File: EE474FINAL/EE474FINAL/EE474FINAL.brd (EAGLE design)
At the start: 69.5 x 84.8 mm, 61 parts, among them U1 TM4C123_DEVICE, U4 3.3V, Y1 32kHz, Y2 Y2

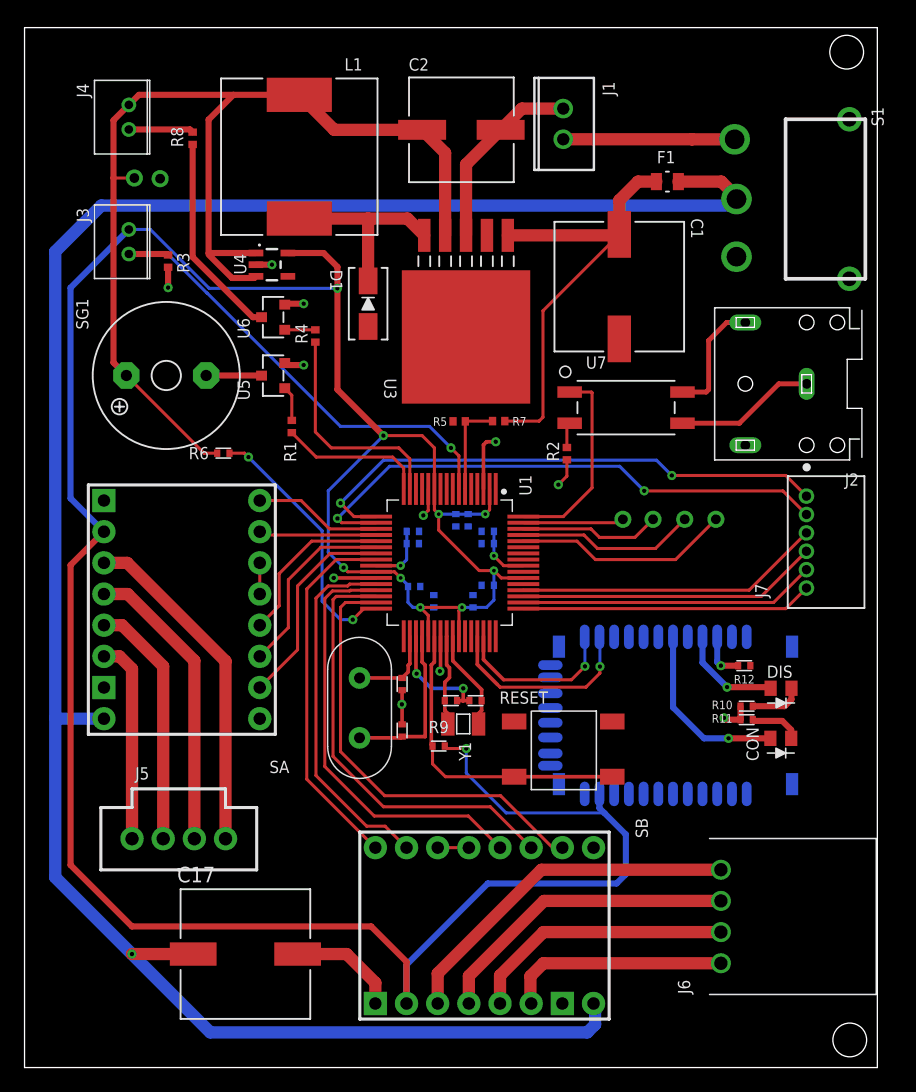
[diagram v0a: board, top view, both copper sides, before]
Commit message: done
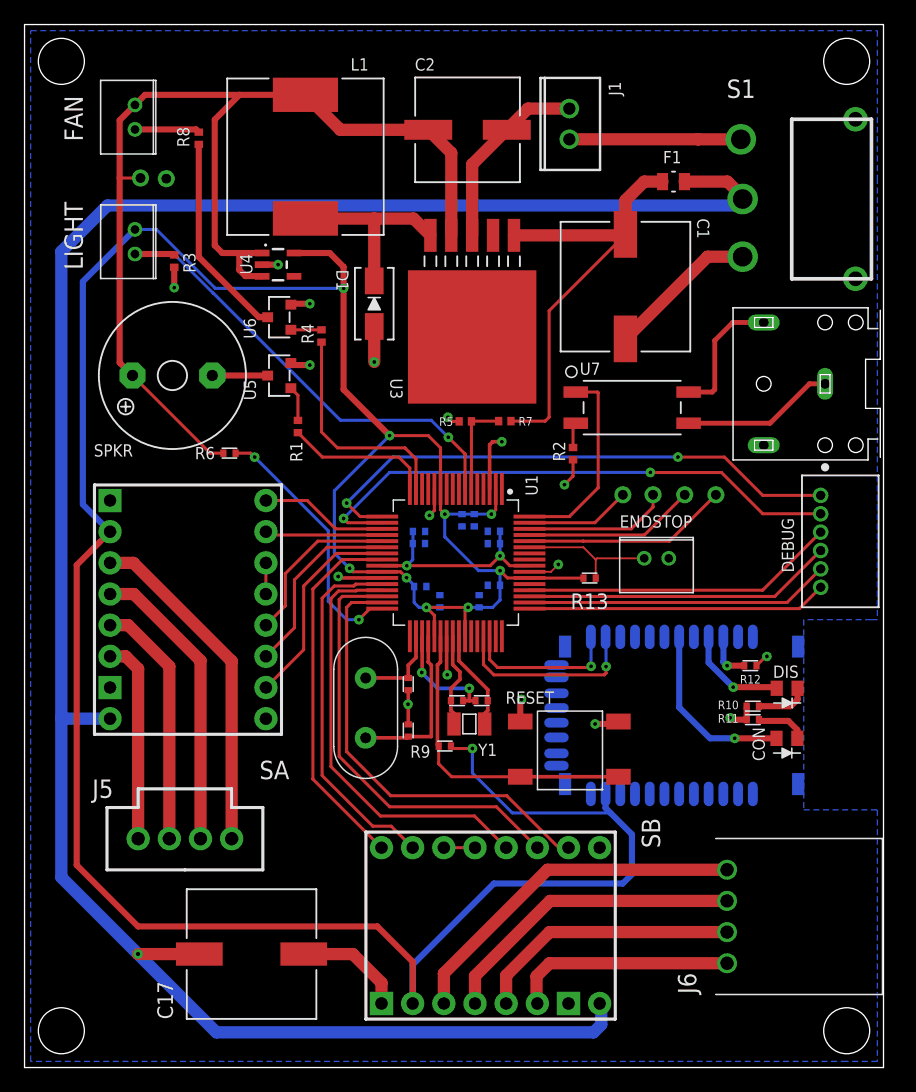
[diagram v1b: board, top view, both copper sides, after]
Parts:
- removed J3, J4: (no value), MICROCONTROLLER:2POS_JSTVERT_2.00
- removed J7: (no value), MICROCONTROLLER:6POS_JST
- removed SG1: F/QMBIII, buzzer:F/QMBIII
- added DEBUG: (no value), MICROCONTROLLER:6POS_JST
- added ENDSTOP, FAN, LIGHT: (no value), MICROCONTROLLER:2POS_JSTVERT_2.00
- added R13: (no value), MICROCONTROLLER:CAPC1005X35N
- added SPKR: F/QMBIII, buzzer:F/QMBIII
- added U$1: (no value), MICROCONTROLLER:LOGO_B
- moved PD0 2.00 mm to (53.8, 46.7)
- moved PD1 2.00 mm to (51.2, 46.7)
- moved PD2 2.00 mm to (48.8, 46.7)
- moved PE5 2.00 mm to (56.3, 46.7)
- moved J2 1.50 mm to (65.2, 55.7)
- moved C1 0.50 mm to (49.0, 63.6)
- moved C10 0.50 mm to (38.3, 42.7)
- moved C11 0.50 mm to (36.6, 44.6)
- moved C12 0.50 mm to (35.6, 44.6)
- moved C13 0.50 mm to (32.2, 39.2)
- moved C14 0.50 mm to (33.9, 38.0)
- moved C15 0.50 mm to (37.0, 38.0)
- moved C16 0.50 mm to (38.2, 39.3)
- moved C17 0.50 mm to (18.5, 9.25)
- moved C2 0.50 mm to (36.1, 76.4)
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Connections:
- new net N$15: ENDSTOP.1, R13.1, U1.59
- net +3V3: now also LIGHT.1, R13.2; no longer J3.1
- net +5V: now also FAN.1, SPKR.+; no longer J4.1, SG1.+
- net FAN_OUT: now also FAN.2; no longer J4.2
- net GND: now also ENDSTOP.2
- net LT: now also LIGHT.2; no longer J3.2
- net N$2: now also SPKR.-; no longer SG1.-
- net RXD: now also DEBUG.6; no longer J7.6
- net TCK: now also DEBUG.4; no longer J7.4
- net TDI: now also DEBUG.2; no longer J7.2
- net TDO: now also DEBUG.1; no longer J7.1
- net TMS: now also DEBUG.3; no longer J7.3
- net TXD: now also DEBUG.5; no longer J7.5
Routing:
- net GND: track 51.7 -> 76.2 mm, vias 11 -> 17
- net N$15: track 0.00 -> 11.3 mm
- net VDDC: track 9.73 -> 17.7 mm
- net +3V3: track 238.0 -> 243.6 mm
- net +5V: track 91.8 -> 90.2 mm
- net N$3: track 9.81 -> 10.8 mm
- net N$4: track 11.5 -> 12.5 mm
- net PE5: track 17.7 -> 16.8 mm
- net RXD: track 44.0 -> 44.8 mm
- net RX-1: track 13.7 -> 12.9 mm
- net TX-0: track 16.5 -> 15.7 mm
- net TMS: track 24.6 -> 25.3 mm
- net TDO: track 23.8 -> 24.4 mm
- net TCK: track 25.0 -> 25.7 mm
- net TDI: track 24.2 -> 24.9 mm
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- added copper zone on layer 16, net GND
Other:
- board size 69.5 x 84.8 mm -> 70 x 85 mm
- board text added: "BRANDON IAMS EE 474 FINAL PROJECT"

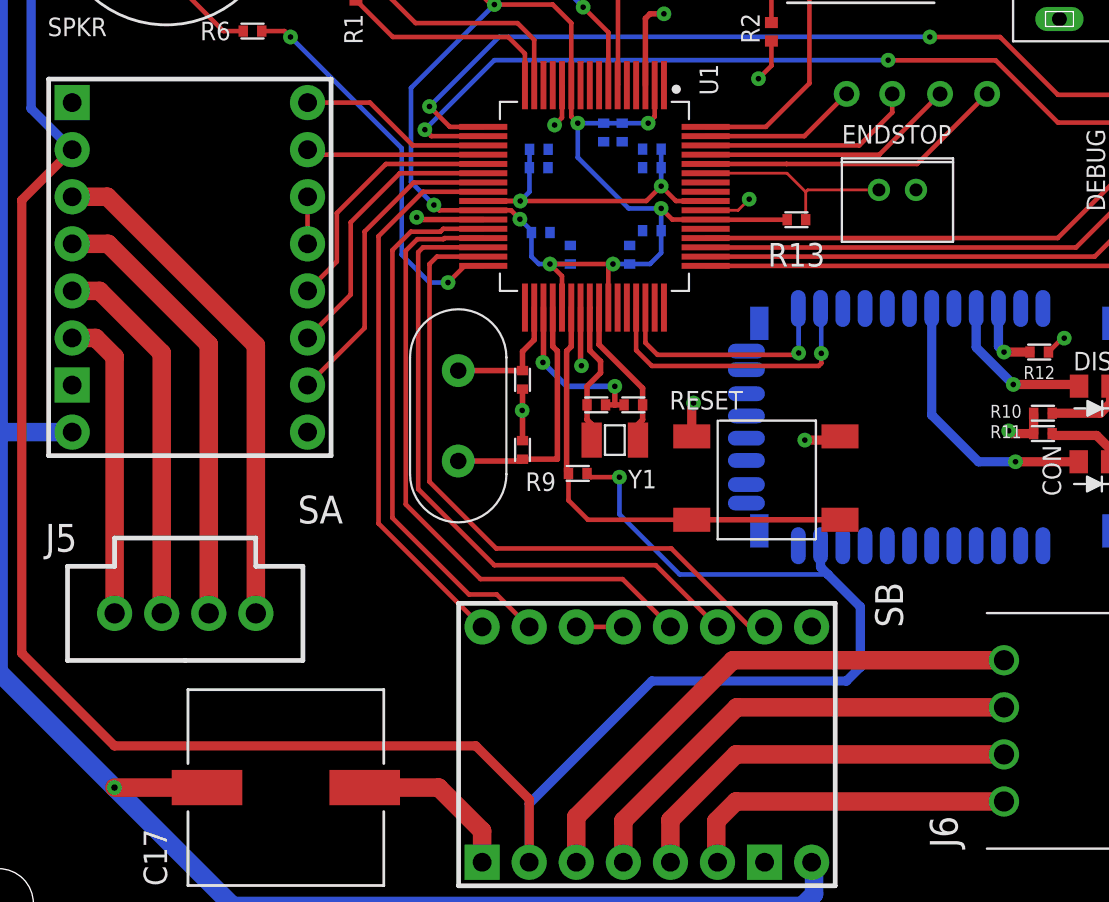
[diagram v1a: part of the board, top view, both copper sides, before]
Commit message: fixing...
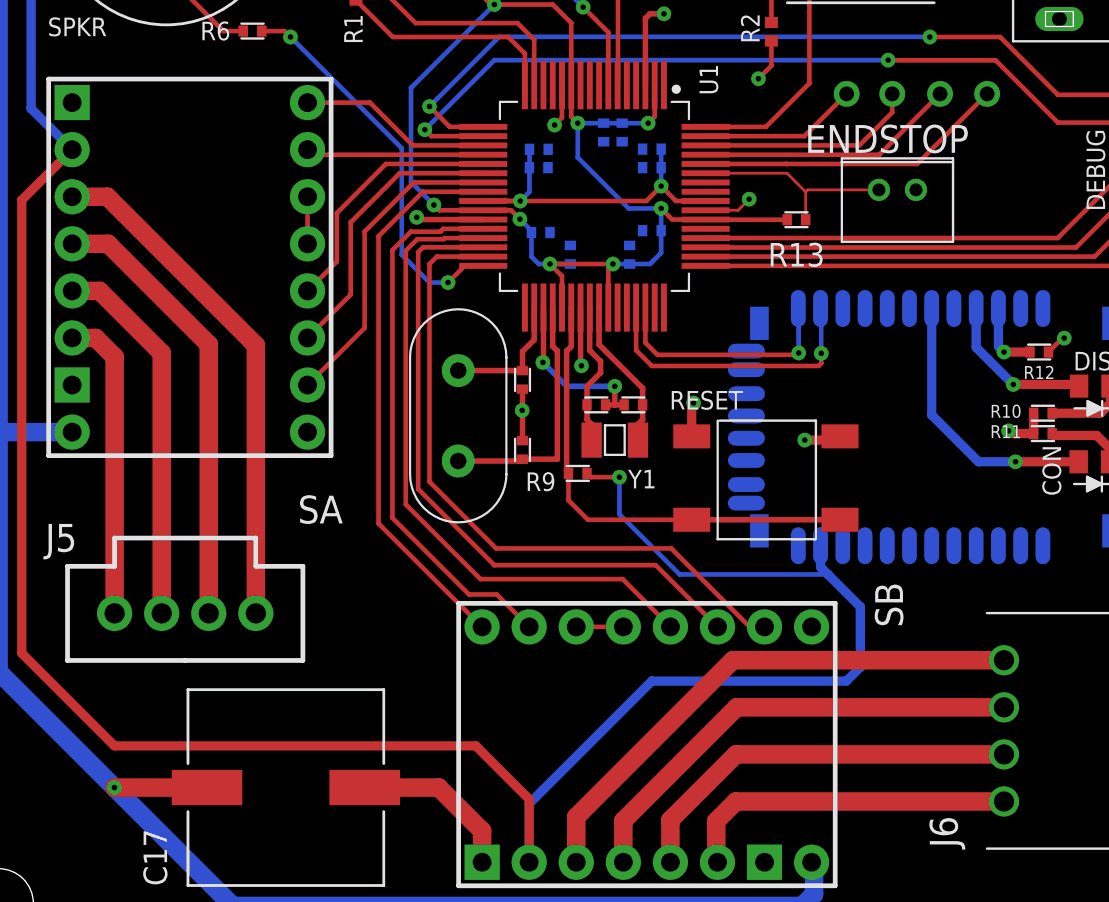
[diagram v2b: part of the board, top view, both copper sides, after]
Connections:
- net GND: now also U3.6

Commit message: merge :
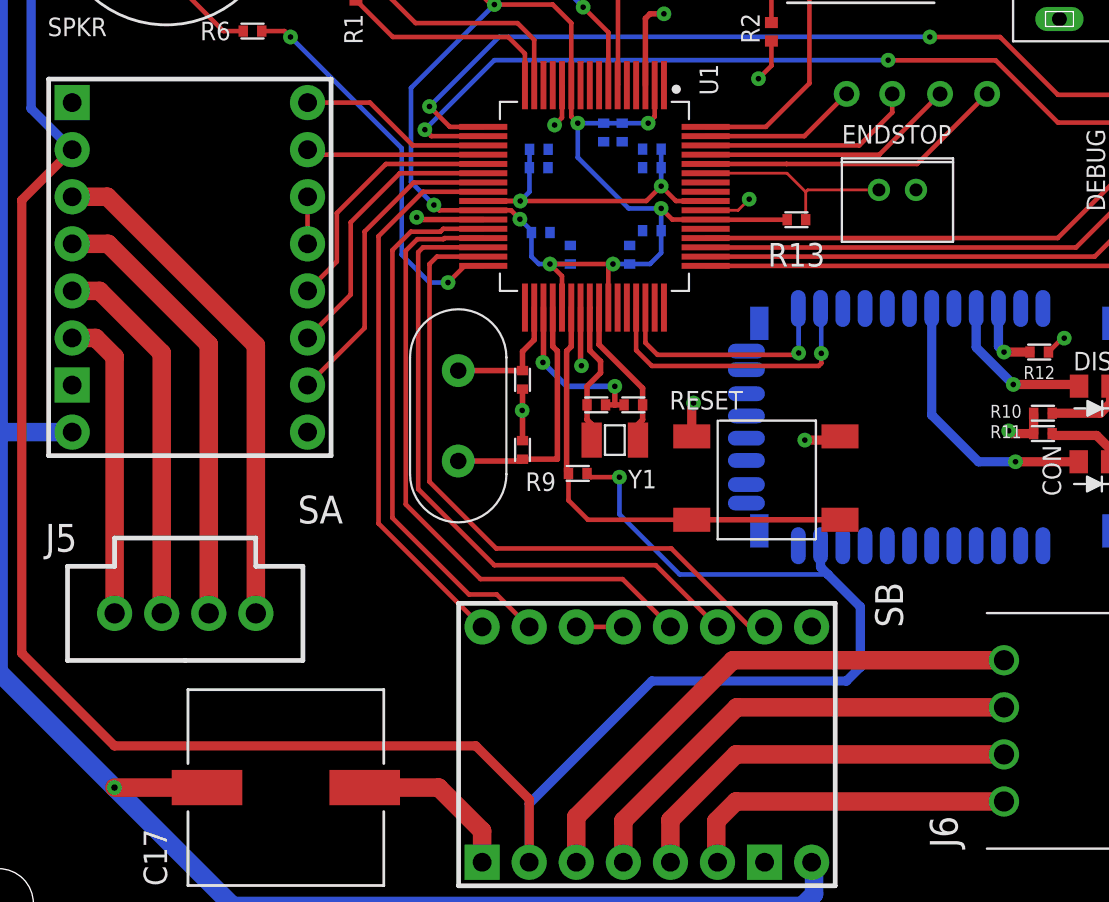
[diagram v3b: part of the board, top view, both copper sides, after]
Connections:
- net GND: no longer U3.6
